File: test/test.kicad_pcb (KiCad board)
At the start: 2 copper layers, 139 x 73.5 mm, 0 parts

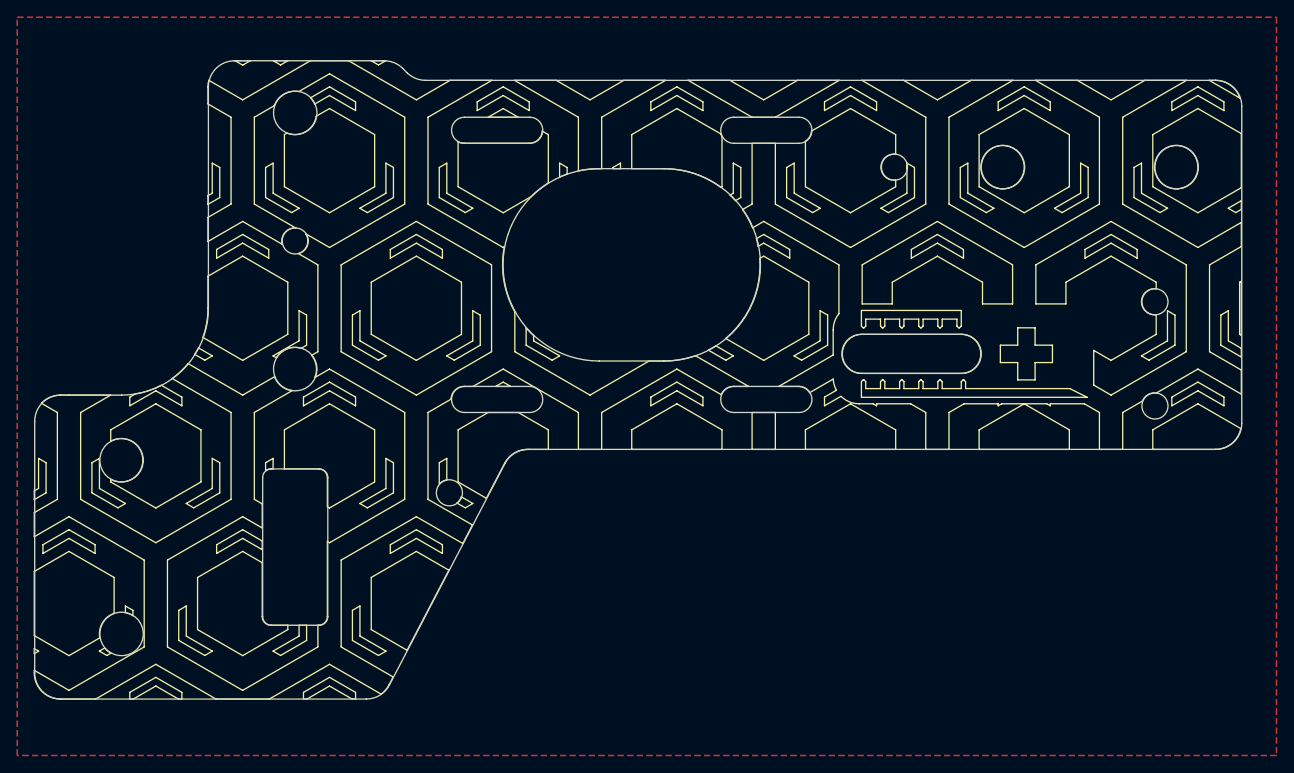
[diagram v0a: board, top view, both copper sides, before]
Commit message: sync
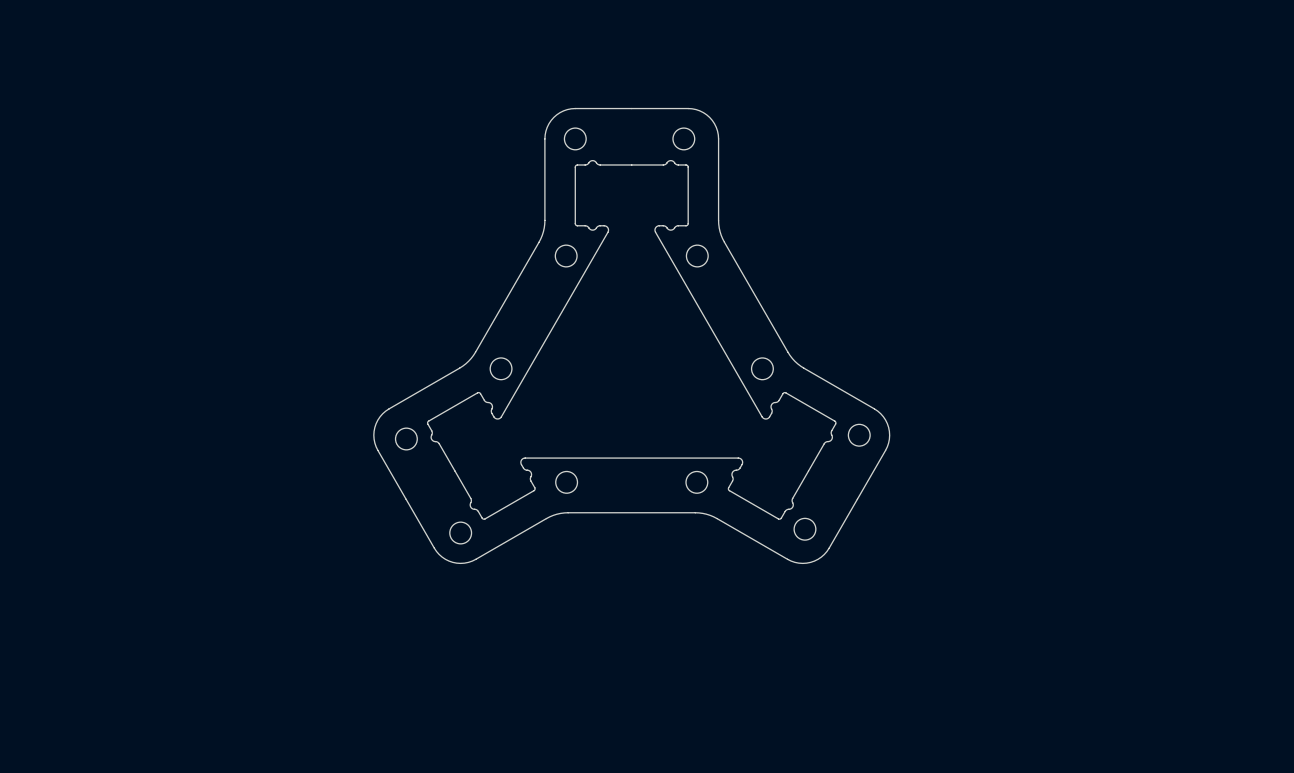
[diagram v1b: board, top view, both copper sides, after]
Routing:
- removed copper zone on F.Cu, net (none)
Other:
- board size 139 x 73.5 mm -> 59.4 x 52.4 mm
